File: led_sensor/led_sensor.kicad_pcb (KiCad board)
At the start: 4 copper layers, 54 parts

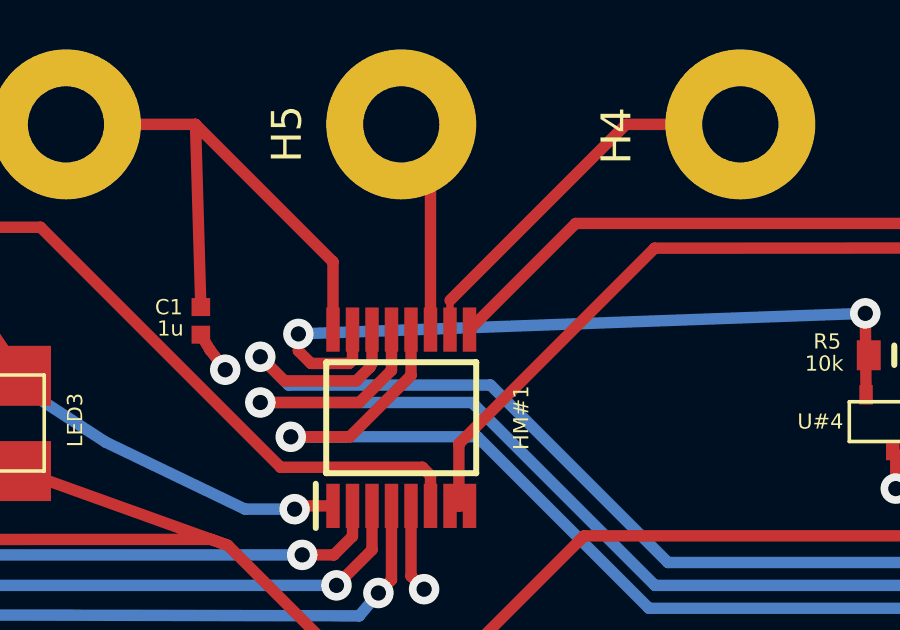
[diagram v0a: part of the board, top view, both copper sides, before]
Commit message: Updated Screenshots
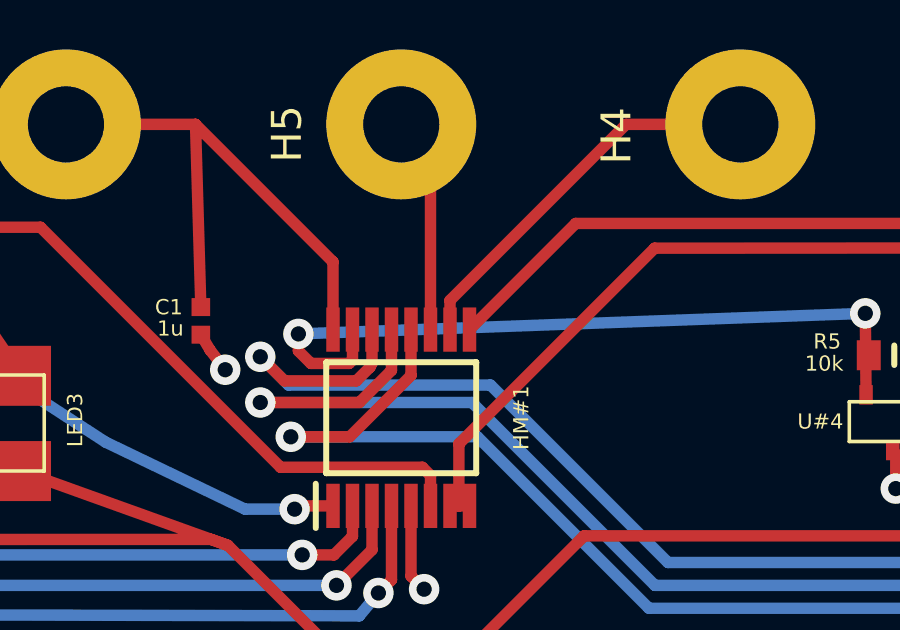
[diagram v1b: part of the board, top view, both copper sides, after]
